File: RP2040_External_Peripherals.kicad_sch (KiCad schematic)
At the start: 28 parts, among them IC1 W25Q16JVSNIQ, J1 Conn_01x03_Pin, Y1 ABM8-272-T3 12MHz

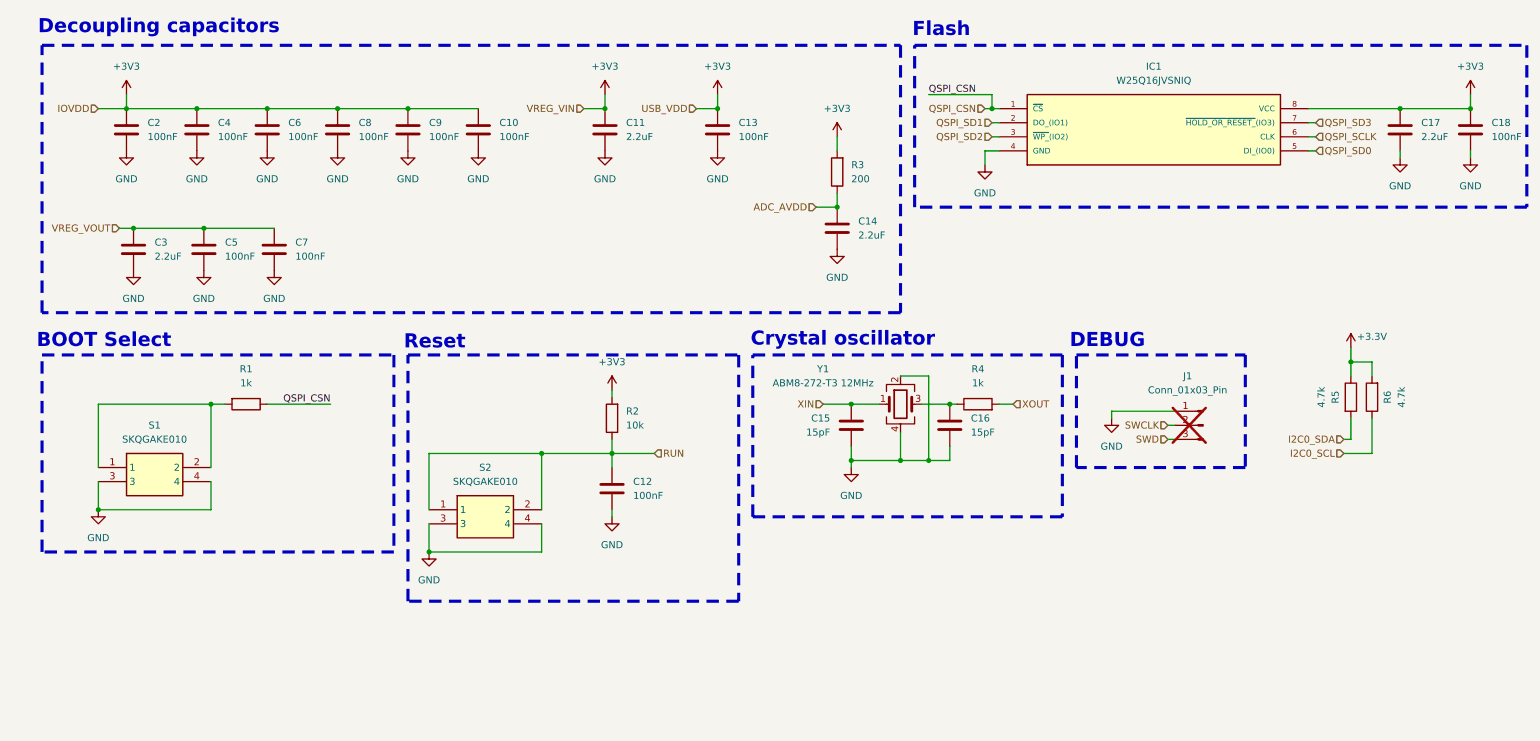
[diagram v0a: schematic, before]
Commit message: Schematic Clean Up
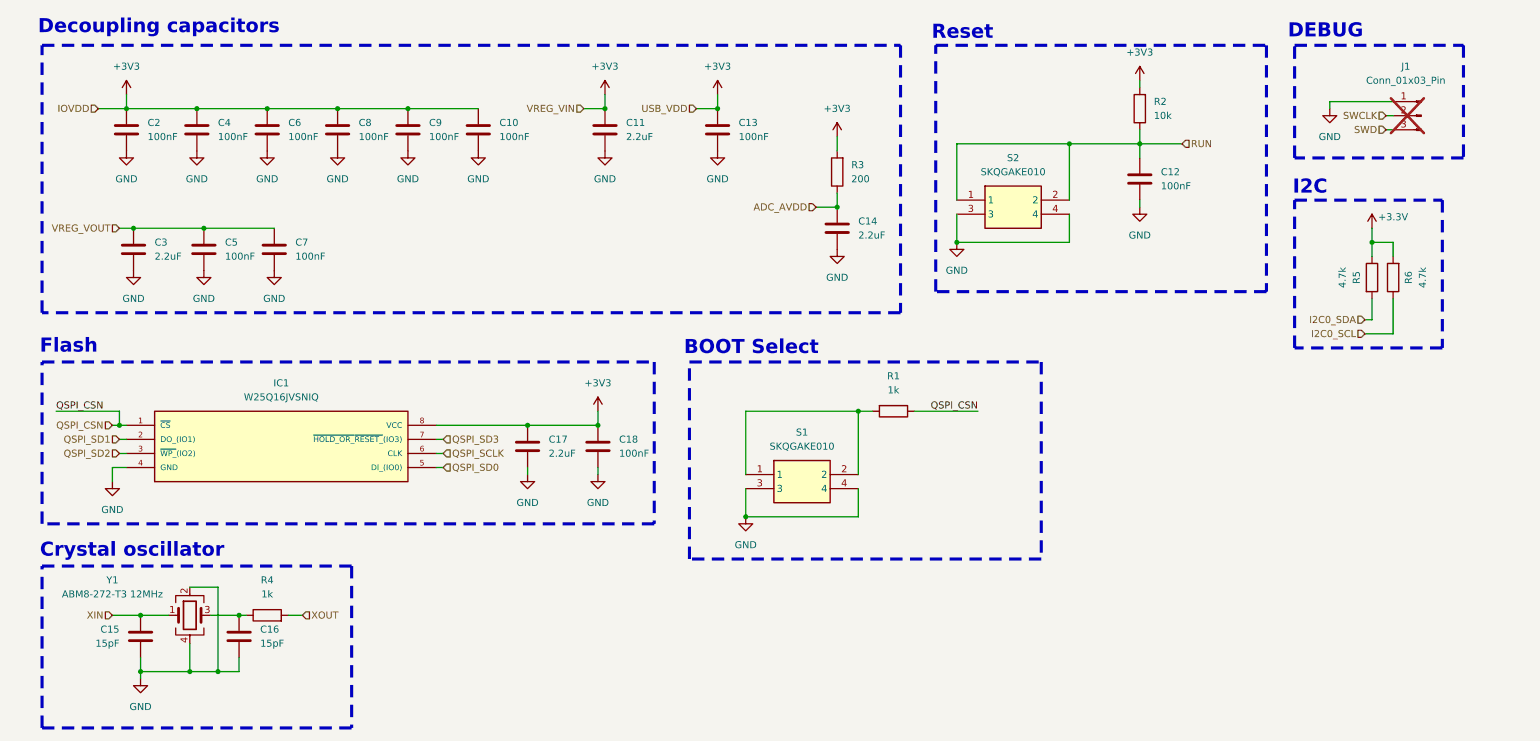
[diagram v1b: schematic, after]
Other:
- note added: "I2C"
- moved on the sheet: C12, C15, C16, C17, C18, IC1, J1, R1, R2, R4, R5, R6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
